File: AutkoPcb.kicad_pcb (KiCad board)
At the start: 2 copper layers, 200 x 120 mm, 45 parts, among them IC201 TEENSY_4.1, J101 Conn_01x06_Male, J102 Conn_01x04_Male, J103 Conn_01x05_Male, J104 Conn_01x04_Male, J105 Conn_01x02_Male, J106 Conn_01x02_Male, J107 Conn_01x02_Male, J108 Conn_01x05_Male, J401 Conn_01x03_Male, J501 Conn_01x03_Male, J601 Conn_01x04_Male, J701 Conn_01x04_Male, J801 Conn_01x04_Male, J901 Screw_Terminal_01x02, SW1001 SW_Push, SW1101 SW_Push, SW1201 SW_Push, SW1301 SW_Push, U901 AZ1117-3.3

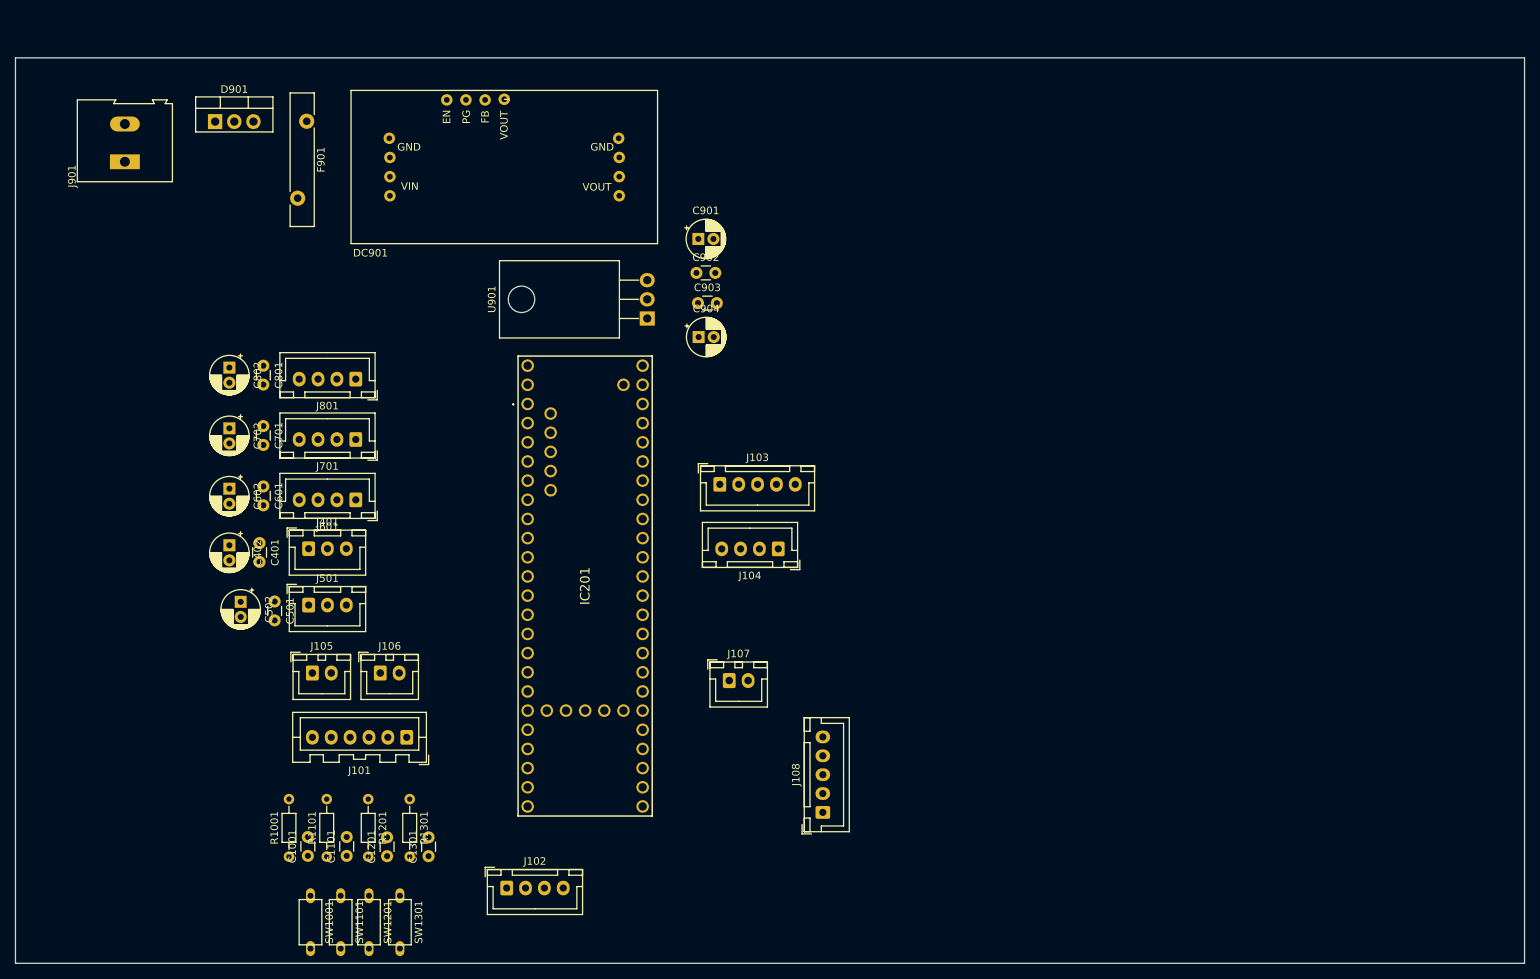
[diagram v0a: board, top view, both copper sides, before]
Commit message: initial PCB layout is done
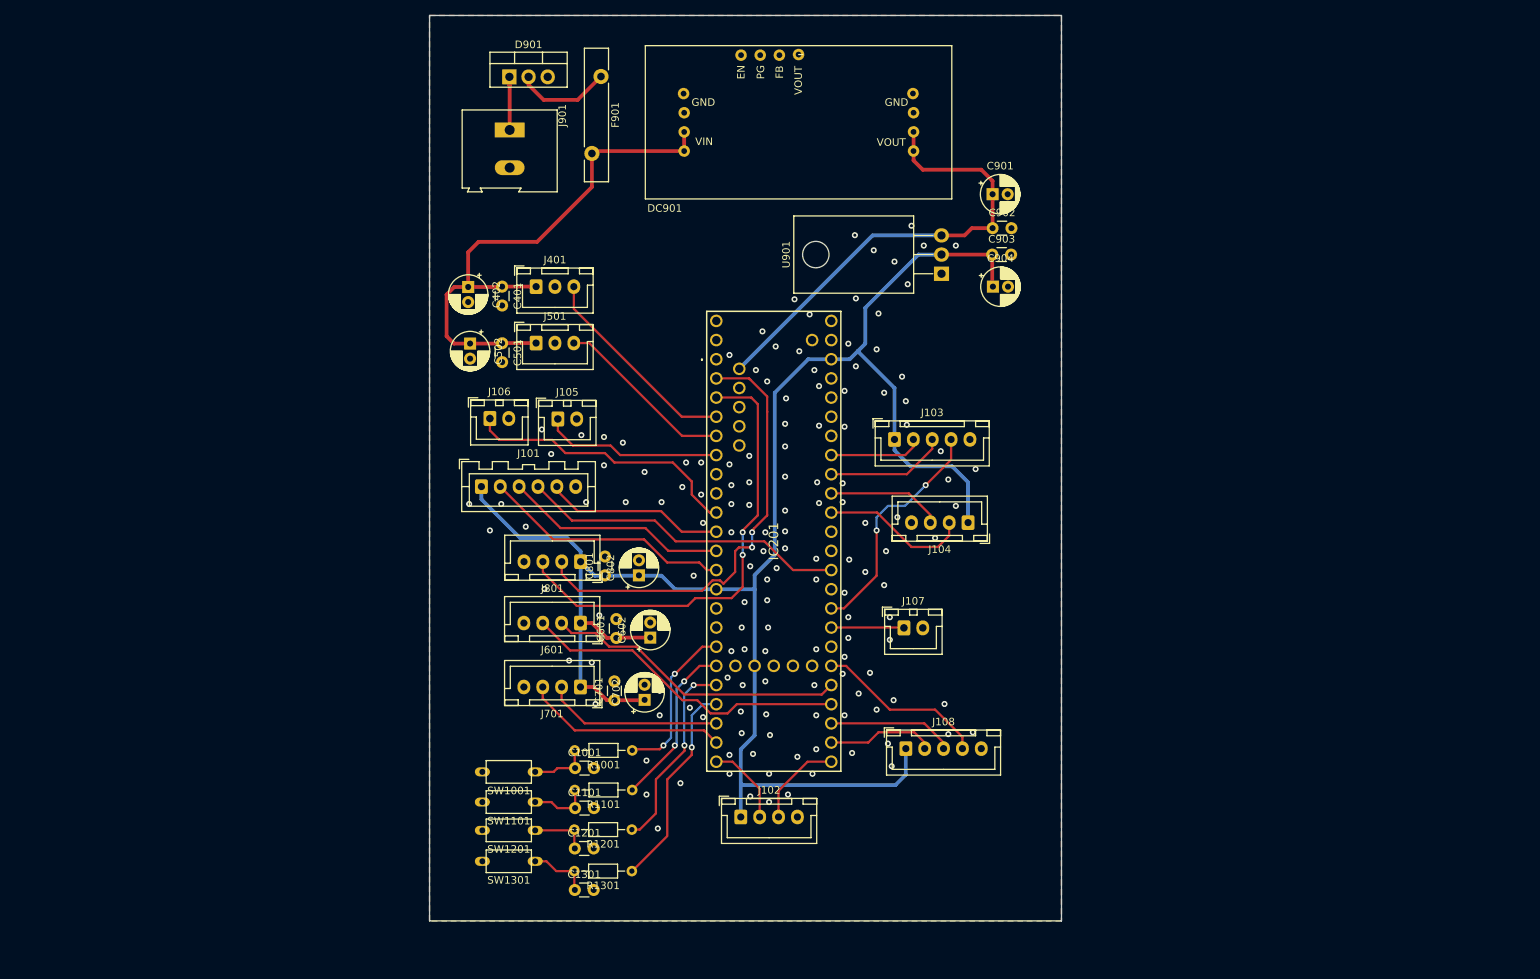
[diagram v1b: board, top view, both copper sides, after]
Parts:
- moved C702 65.8 mm to (127.4, 121.1), turned to 90 degrees
- moved C802 60.9 mm to (126.6, 104.6), turned to 90 degrees
- moved C602 59.2 mm to (128.1, 112.8), turned to 90 degrees
- moved C701 59.0 mm to (123.4, 121.1), turned to 90 degrees
- moved C801 53.1 mm to (122.1, 104.6), turned to 90 degrees
- moved J901 51.2 mm to (109.5, 45.6), turned to -90 degrees
- moved C601 50.9 mm to (123.6, 112.9), turned to 90 degrees
- moved R1001 47.6 mm to (125.7, 127.8), turned to 180 degrees
- moved J105 46.8 mm to (115.9, 83.9)
- moved C401 46.8 mm to (108.5, 66.3)
- moved C402 46.6 mm to (104.0, 66.4)
- moved J401 46.0 mm to (113.0, 66.3)
- moved J501 46.0 mm to (113.0, 73.8)
- moved C502 45.8 mm to (104.2, 73.9)
- moved C501 45.6 mm to (108.5, 73.8)
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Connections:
- net Net-(D901-Pad1) renamed /Power/VIN_CONN
- net Net-(D901-Pad2) renamed /Power/VIN_FUSE
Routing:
- net +3.3V: track 0.00 -> 239.2 mm
- net VCC: track 0.00 -> 74.0 mm
- net +5V: track 0.00 -> 62.9 mm
- net /ULTRAD3_B: track 0.00 -> 61.7 mm, vias 0 -> 2
- net /ULTRAD3_A: track 0.00 -> 60.7 mm, vias 0 -> 2
- net /ULTRAD1_B: track 0.00 -> 43.7 mm
- net /DISP_SCK: track 0.00 -> 43.5 mm
- net /ULTRAD1_A: track 0.00 -> 40.2 mm
- net /STEERING: track 0.00 -> 37.1 mm
- net /DISP_MISO: track 0.00 -> 33.2 mm
- net /TOF_INT: track 0.00 -> 31.3 mm, vias 0 -> 2
- net /DISP_MOSI: track 0.00 -> 29.7 mm
- net /BUTTON_D: track 0.00 -> 27.8 mm, vias 0 -> 1
- net /CAMERA_SERVO_A: track 0.00 -> 27.7 mm
- net /ULTRAD2_B: track 0.00 -> 26.9 mm
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- added copper zone on B.Cu, net GND
- added copper zone on F.Cu, net GND
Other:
- board size 200 x 120 mm -> 83.8 x 120 mm
